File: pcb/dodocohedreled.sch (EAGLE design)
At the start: 11 parts

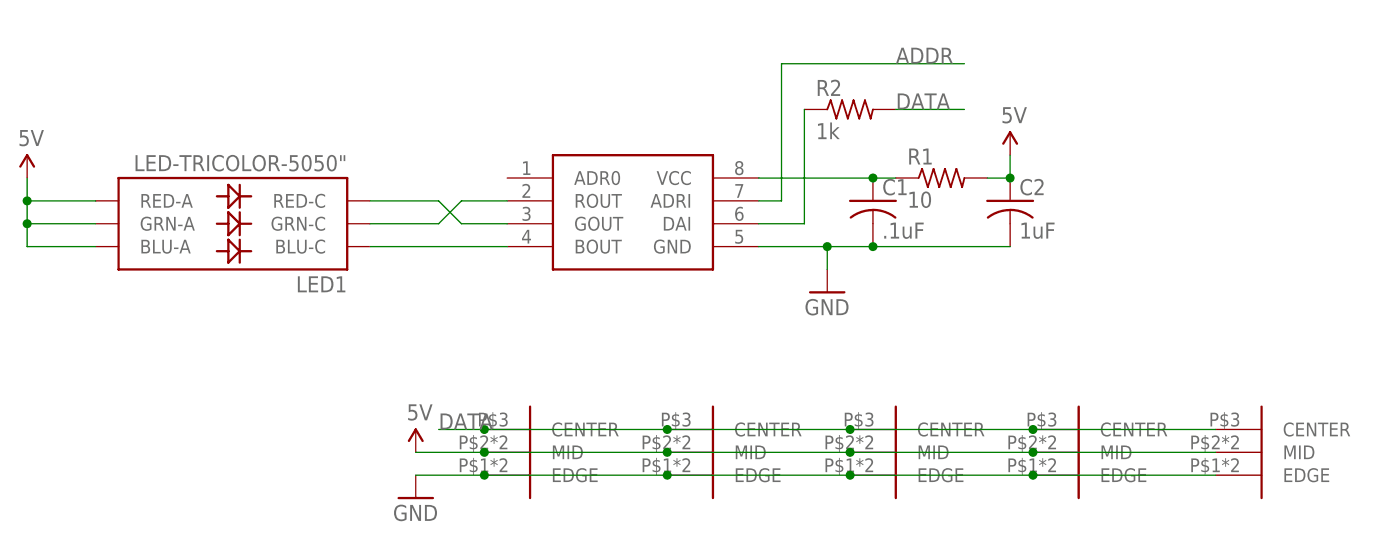
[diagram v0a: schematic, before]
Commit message: Update for RevC
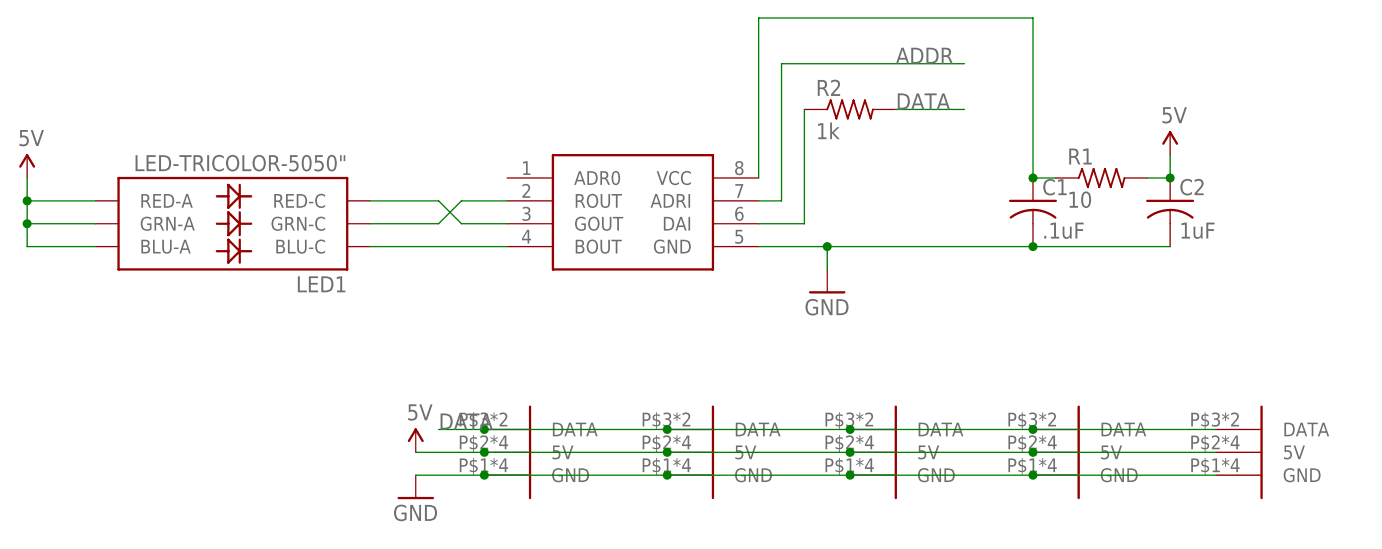
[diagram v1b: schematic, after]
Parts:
- U$2, U$3, U$4, U$5, U$6: value D_EDGE -> D_EDGESLOT; device dodocohedreled:D_EDGE -> dodocohedreled:D_EDGESLOT
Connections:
- net 5V: now also U$2.5V, U$3.5V, U$4.5V, U$5.5V, U$6.5V; no longer U$2.MID, U$3.MID, U$4.MID, U$5.MID, U$6.MID
- net DATA: now also U$2.DATA, U$3.DATA, U$4.DATA, U$5.DATA, U$6.DATA; no longer U$2.CENTER, U$3.CENTER, U$4.CENTER, U$5.CENTER, U$6.CENTER
- net GND: now also U$2.GND, U$3.GND, U$4.GND, U$5.GND, U$6.GND; no longer U$2.EDGE, U$3.EDGE, U$4.EDGE, U$5.EDGE, U$6.EDGE
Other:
- moved on the sheet: C1, C2, R1
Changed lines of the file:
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@@
 <part name="R2" library="adafruit" deviceset="R-US_" device="R0603" value="1k"/>
 <part name="SUPPLY2" library="SparkFun-Aesthetics" deviceset="5V" device=""/>
-<part name="U$2" library="dodocohedreled" deviceset="D_EDGE" device=""/>
+<part name="U$2" library="dodocohedreled" deviceset="D_EDGE" device="SLOT"/>
 <part name="SUPPLY3" library="SparkFun-Aesthetics" deviceset="5V" device=""/>
 <part name="GND2" library="SparkFun-Aesthetics" deviceset="GND" device=""/>
-<part name="U$3" library="dodocohedreled" deviceset="D_EDGE" device=""/>
-<part name="U$4" library="dodocohedreled" deviceset="D_EDGE" device=""/>
-<part name="U$5" library="dodocohedreled" deviceset="D_EDGE" device=""/>
-<part name="U$6" library="dodocohedreled" deviceset="D_EDGE" device=""/>
+<part name="U$3" library="dodocohedreled" deviceset="D_EDGE" device="SLOT"/>
+<part name="U$4" library="dodocohedreled" deviceset="D_EDGE" device="SLOT"/>
+<part name="U$5" library="dodocohedreled" deviceset="D_EDGE" device="SLOT"/>
+<part name="U$6" library="dodocohedreled" deviceset="D_EDGE" device="SLOT"/>
 </parts>
 <sheets>
@@
 <instance part="GND1" gate="1" x="81.28" y="73.66"/>
 <instance part="U$1" gate="G$1" x="53.34" y="81.28"/>
-<instance part="C1" gate="G$1" x="86.36" y="83.82"/>
-<instance part="C2" gate="G$1" x="101.6" y="83.82"/>
-<instance part="R1" gate="G$1" x="93.98" y="86.36"/>
+<instance part="C1" gate="G$1" x="104.14" y="83.82"/>
+<instance part="C2" gate="G$1" x="119.38" y="83.82"/>
+<instance part="R1" gate="G$1" x="111.76" y="86.36"/>
 <instance part="R2" gate="G$1" x="83.82" y="93.98"/>
-<instance part="SUPPLY2" gate="G$1" x="101.6" y="88.9"/>
+<instance part="SUPPLY2" gate="G$1" x="119.38" y="88.9"/>
 <instance part="U$2" gate="G$1" x="124.46" y="58.42"/>
 <instance part="SUPPLY3" gate="G$1" x="35.56" y="55.88"/>
@@
 <pinref part="R1" gate="G$1" pin="2"/>
 <pinref part="C2" gate="G$1" pin="1"/>
-<wire x1="99.06" y1="86.36" x2="101.6" y2="86.36" width="0.1524" layer="91"/>
+<wire x1="116.84" y1="86.36" x2="119.38" y2="86.36" width="0.1524" layer="91"/>
 <pinref part="SUPPLY2" gate="G$1" pin="5V"/>
-<wire x1="101.6" y1="88.9" x2="101.6" y2="86.36" width="0.1524" layer="91"/>
-<junction x="101.6" y="86.36"/>
+<wire x1="119.38" y1="88.9" x2="119.38" y2="86.36" width="0.1524" layer="91"/>
+<junction x="119.38" y="86.36"/>
 </segment>
 <segment>
-<pinref part="U$2" gate="G$1" pin="MID"/>
+<pinref part="U$2" gate="G$1" pin="5V"/>
 <wire x1="124.46" y1="55.88" x2="104.14" y2="55.88" width="0.1524" layer="91"/>
 <pinref part="SUPPLY3" gate="G$1" pin="5V"/>
-<pinref part="U$3" gate="G$1" pin="MID"/>
+<pinref part="U$3" gate="G$1" pin="5V"/>
 <wire x1="104.14" y1="55.88" x2="83.82" y2="55.88" width="0.1524" layer="91"/>
 <wire x1="83.82" y1="55.88" x2="63.5" y2="55.88" width="0.1524" layer="91"/>
 <wire x1="63.5" y1="55.88" x2="43.18" y2="55.88" width="0.1524" layer="91"/>
 <junction x="63.5" y="55.88"/>
-<pinref part="U$4" gate="G$1" pin="MID"/>
+<pinref part="U$4" gate="G$1" pin="5V"/>
 <wire x1="43.18" y1="55.88" x2="35.56" y2="55.88" width="0.1524" layer="91"/>
 <junction x="43.18" y="55.88"/>
-<pinref part="U$5" gate="G$1" pin="MID"/>
+<pinref part="U$5" gate="G$1" pin="5V"/>
 <junction x="83.82" y="55.88"/>
-<pinref part="U$6" gate="G$1" pin="MID"/>
+<pinref part="U$6" gate="G$1" pin="5V"/>
 <junction x="104.14" y="55.88"/>
 </segment>
@@
 <pinref part="C2" gate="G$1" pin="2"/>
 <pinref part="C1" gate="G$1" pin="2"/>
-<wire x1="101.6" y1="78.74" x2="86.36" y2="78.74" width="0.1524" layer="91"/>
-<wire x1="86.36" y1="78.74" x2="81.28" y2="78.74" width="0.1524" layer="91"/>
+<wire x1="119.38" y1="78.74" x2="104.14" y2="78.74" width="0.1524" layer="91"/>
+<wire x1="104.14" y1="78.74" x2="81.28" y2="78.74" width="0.1524" layer="91"/>
 <junction x="81.28" y="78.74"/>
-<junction x="86.36" y="78.74"/>
+<junction x="104.14" y="78.74"/>
 </segment>
 <segment>
-<pinref part="U$2" gate="G$1" pin="EDGE"/>
+<pinref part="U$2" gate="G$1" pin="GND"/>
 <wire x1="124.46" y1="53.34" x2="104.14" y2="53.34" width="0.1524" layer="91"/>
 <pinref part="GND2" gate="1" pin="GND"/>
-<pinref part="U$3" gate="G$1" pin="EDGE"/>
+<pinref part="U$3" gate="G$1" pin="GND"/>
 <wire x1="104.14" y1="53.34" x2="83.82" y2="53.34" width="0.1524" layer="91"/>
 <wire x1="83.82" y1="53.34" x2="63.5" y2="53.34" width="0.1524" layer="91"/>
 <wire x1="63.5" y1="53.34" x2="43.18" y2="53.34" width="0.1524" layer="91"/>
 <junction x="63.5" y="53.34"/>
-<pinref part="U$4" gate="G$1" pin="EDGE"/>
+<pinref part="U$4" gate="G$1" pin="GND"/>
 <wire x1="43.18" y1="53.34" x2="35.56" y2="53.34" width="0.1524" layer="91"/>
 <junction x="43.18" y="53.34"/>
-<pinref part="U$5" gate="G$1" pin="EDGE"/>
+<pinref part="U$5" gate="G$1" pin="GND"/>
 <junction x="83.82" y="53.34"/>
-<pinref part="U$6" gate="G$1" pin="EDGE"/>
+<pinref part="U$6" gate="G$1" pin="GND"/>
 <junction x="104.14" y="53.34"/>
 </segment>
@@
 <pinref part="U$1" gate="G$1" pin="VCC"/>
 <pinref part="C1" gate="G$1" pin="1"/>
-<wire x1="73.66" y1="86.36" x2="86.36" y2="86.36" width="0.1524" layer="91"/>
+<wire x1="73.66" y1="86.36" x2="73.66" y2="104.14" width="0.1524" layer="91"/>
+<wire x1="73.66" y1="104.14" x2="104.14" y2="104.14" width="0.1524" layer="91"/>
+<wire x1="104.14" y1="104.14" x2="104.14" y2="86.36" width="0.1524" layer="91"/>
 <pinref part="R1" gate="G$1" pin="1"/>
-<wire x1="86.36" y1="86.36" x2="88.9" y2="86.36" width="0.1524" layer="91"/>
-<junction x="86.36" y="86.36"/>
+<wire x1="104.14" y1="86.36" x2="106.68" y2="86.36" width="0.1524" layer="91"/>
+<junction x="104.14" y="86.36"/>
 </segment>
 </net>
@@
 </segment>
 <segment>
-<pinref part="U$2" gate="G$1" pin="CENTER"/>
+<pinref part="U$2" gate="G$1" pin="DATA"/>
 <wire x1="124.46" y1="58.42" x2="104.14" y2="58.42" width="0.1524" layer="91"/>
 <label x="38.1" y="58.42" size="1.778" layer="95"/>
-<pinref part="U$3" gate="G$1" pin="CENTER"/>
+<pinref part="U$3" gate="G$1" pin="DATA"/>
 <wire x1="104.14" y1="58.42" x2="83.82" y2="58.42" width="0.1524" layer="91"/>
 <wire x1="83.82" y1="58.42" x2="63.5" y2="58.42" width="0.1524" layer="91"/>
 <wire x1="63.5" y1="58.42" x2="43.18" y2="58.42" width="0.1524" layer="91"/>
 <junction x="63.5" y="58.42"/>
-<pinref part="U$4" gate="G$1" pin="CENTER"/>
+<pinref part="U$4" gate="G$1" pin="DATA"/>
 <wire x1="43.18" y1="58.42" x2="38.1" y2="58.42" width="0.1524" layer="91"/>
 <junction x="43.18" y="58.42"/>
-<pinref part="U$5" gate="G$1" pin="CENTER"/>
+<pinref part="U$5" gate="G$1" pin="DATA"/>
 <junction x="83.82" y="58.42"/>
-<pinref part="U$6" gate="G$1" pin="CENTER"/>
+<pinref part="U$6" gate="G$1" pin="DATA"/>
 <junction x="104.14" y="58.42"/>
 </segment>
